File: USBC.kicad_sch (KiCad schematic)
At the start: 17 parts, among them J5 USB_C_Receptacle, U11 FUSB302BMPX, U12 TPD4E05U06DQA, U13 TPD4E05U06DQA

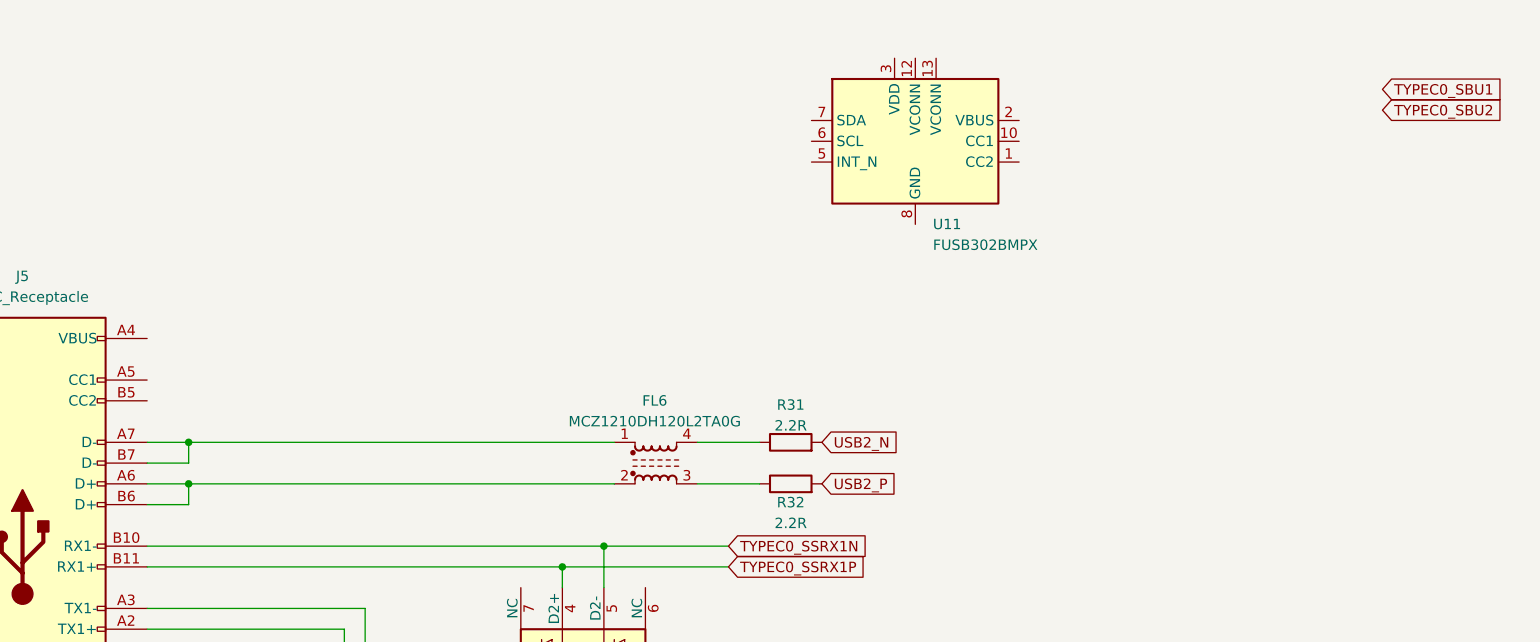
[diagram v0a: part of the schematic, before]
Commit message: usbc work
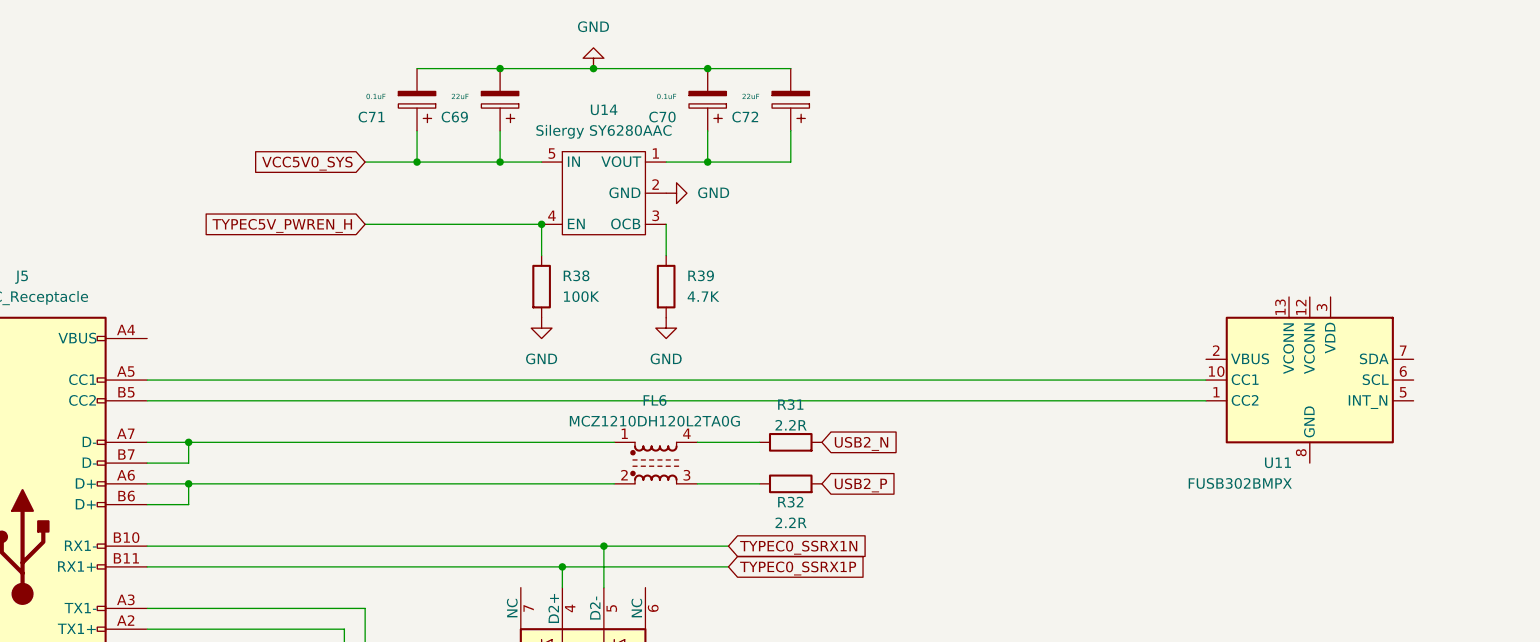
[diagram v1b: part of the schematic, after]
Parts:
- added C69, C72: 22uF, symbol Device:C_Polarized
- added C70, C71: 0.1uF, symbol Device:C_Polarized
- added R38: 100K, symbol Device:R
- added R39: 4.7K, symbol Device:R
- added U14: Silergy SY6280AAC, symbol raxda:SGM2576YN5G/TR
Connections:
- net GND: now also C69.2, C70.2, C71.2, C72.2, R38.2, R39.2, U14.2 (GND)
- net at J5.A5 (CC1): now also U11.10 (CC1), U11.11 (CC1)
- net at J5.B5 (CC2): now also U11.1 (CC2), U11.14 (CC2)
- new net: R39.1, U14.3 (OCB)
- new net: C70.1, C72.1, U14.1 (VOUT)
- new net TYPEC5V_PWREN_H: R38.1, U14.4 (EN)
- new net VCC5V0_SYS: C69.1, C71.1, U14.5 (IN)
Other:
- moved on the sheet: U11
